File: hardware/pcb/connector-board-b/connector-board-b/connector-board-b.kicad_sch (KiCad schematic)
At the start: 44 parts, among them J1 DE9_Pins, J2 PANEL_18V, J5 8-215570-0, J6 NTC_103AT, J7 BATTERY, Q1 Si4840BDY, Q2 Si4840BDY, SW1 PWR_KILL, U1 BQ24650RVA, U2 INA3221, U3 MCP1700-3.3

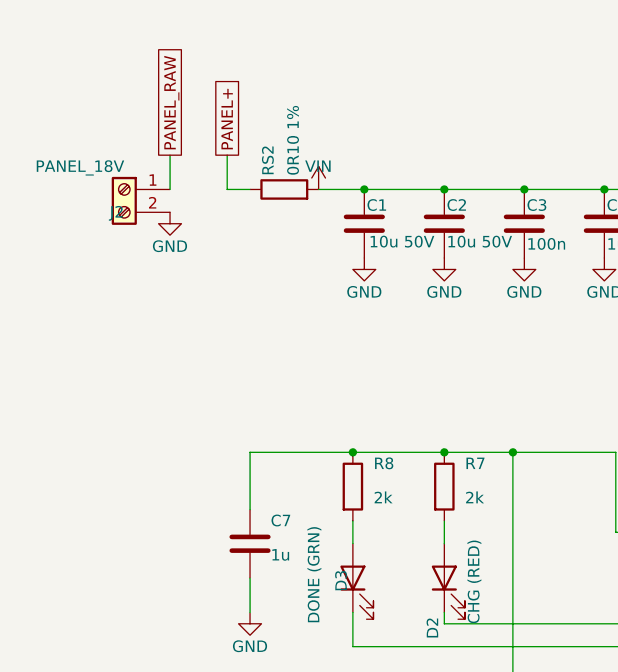
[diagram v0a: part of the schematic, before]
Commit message: Misc changes
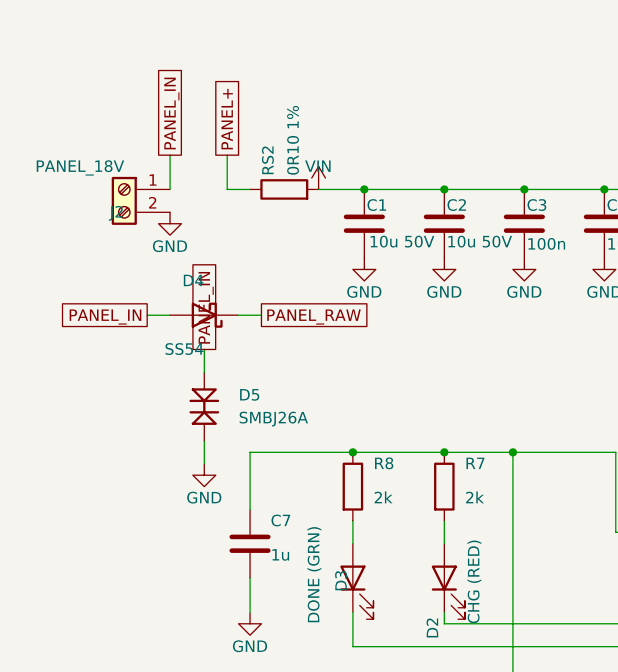
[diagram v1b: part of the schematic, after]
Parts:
- added D4: SS54, Diode_SMD:D_SMA, symbol Device:D_Schottky
- added D5: SMBJ26A, Diode_SMD:D_SMB, symbol lora3v3:TVS_V
- L1: LCSC Part # C511353 -> C845066
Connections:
- net GND: now also D5.2
- net PANEL_RAW: now also D4.1 (K); no longer J2.1 (Pin_1)
- new net PANEL_IN: D4.2 (A), D5.1, J2.1 (Pin_1)
